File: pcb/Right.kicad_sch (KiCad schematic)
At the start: 51 parts

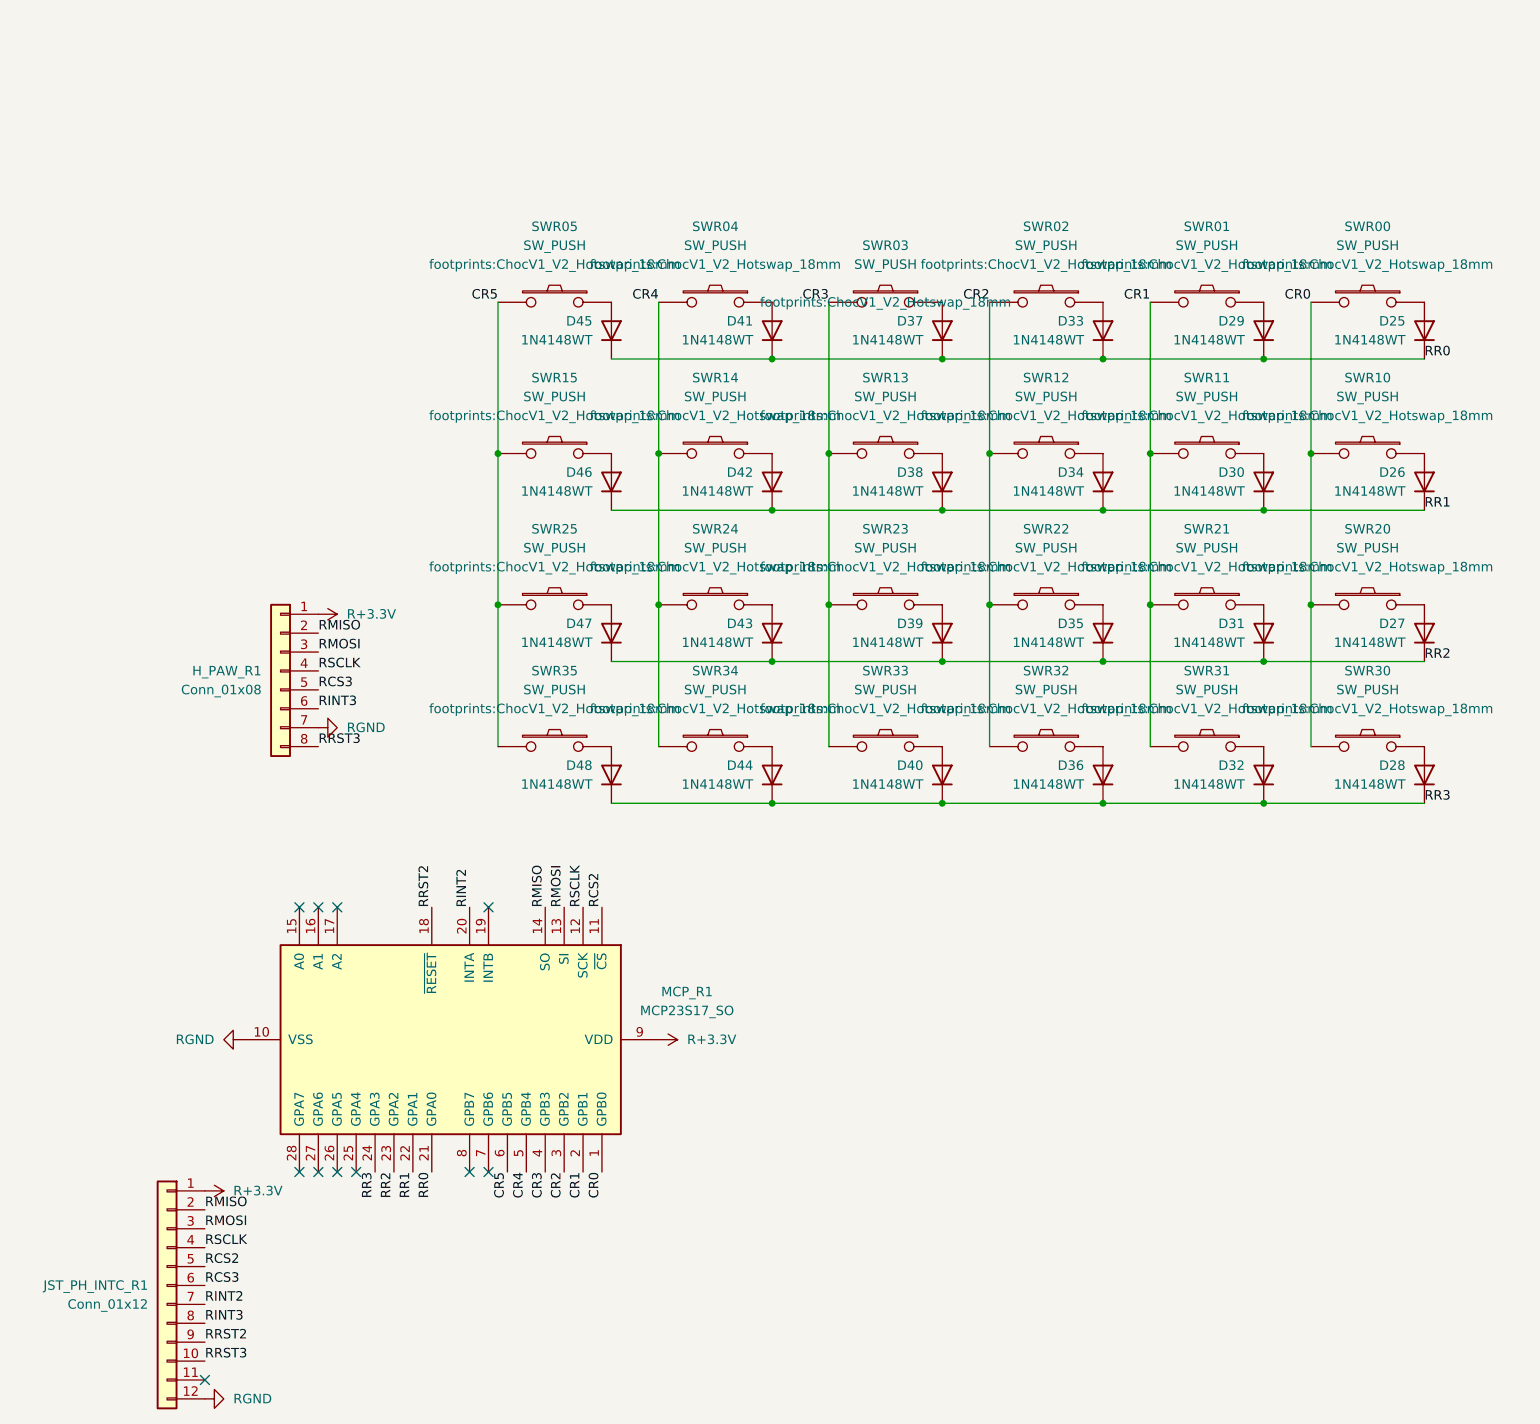
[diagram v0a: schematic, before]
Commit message: Clean up folder structure.
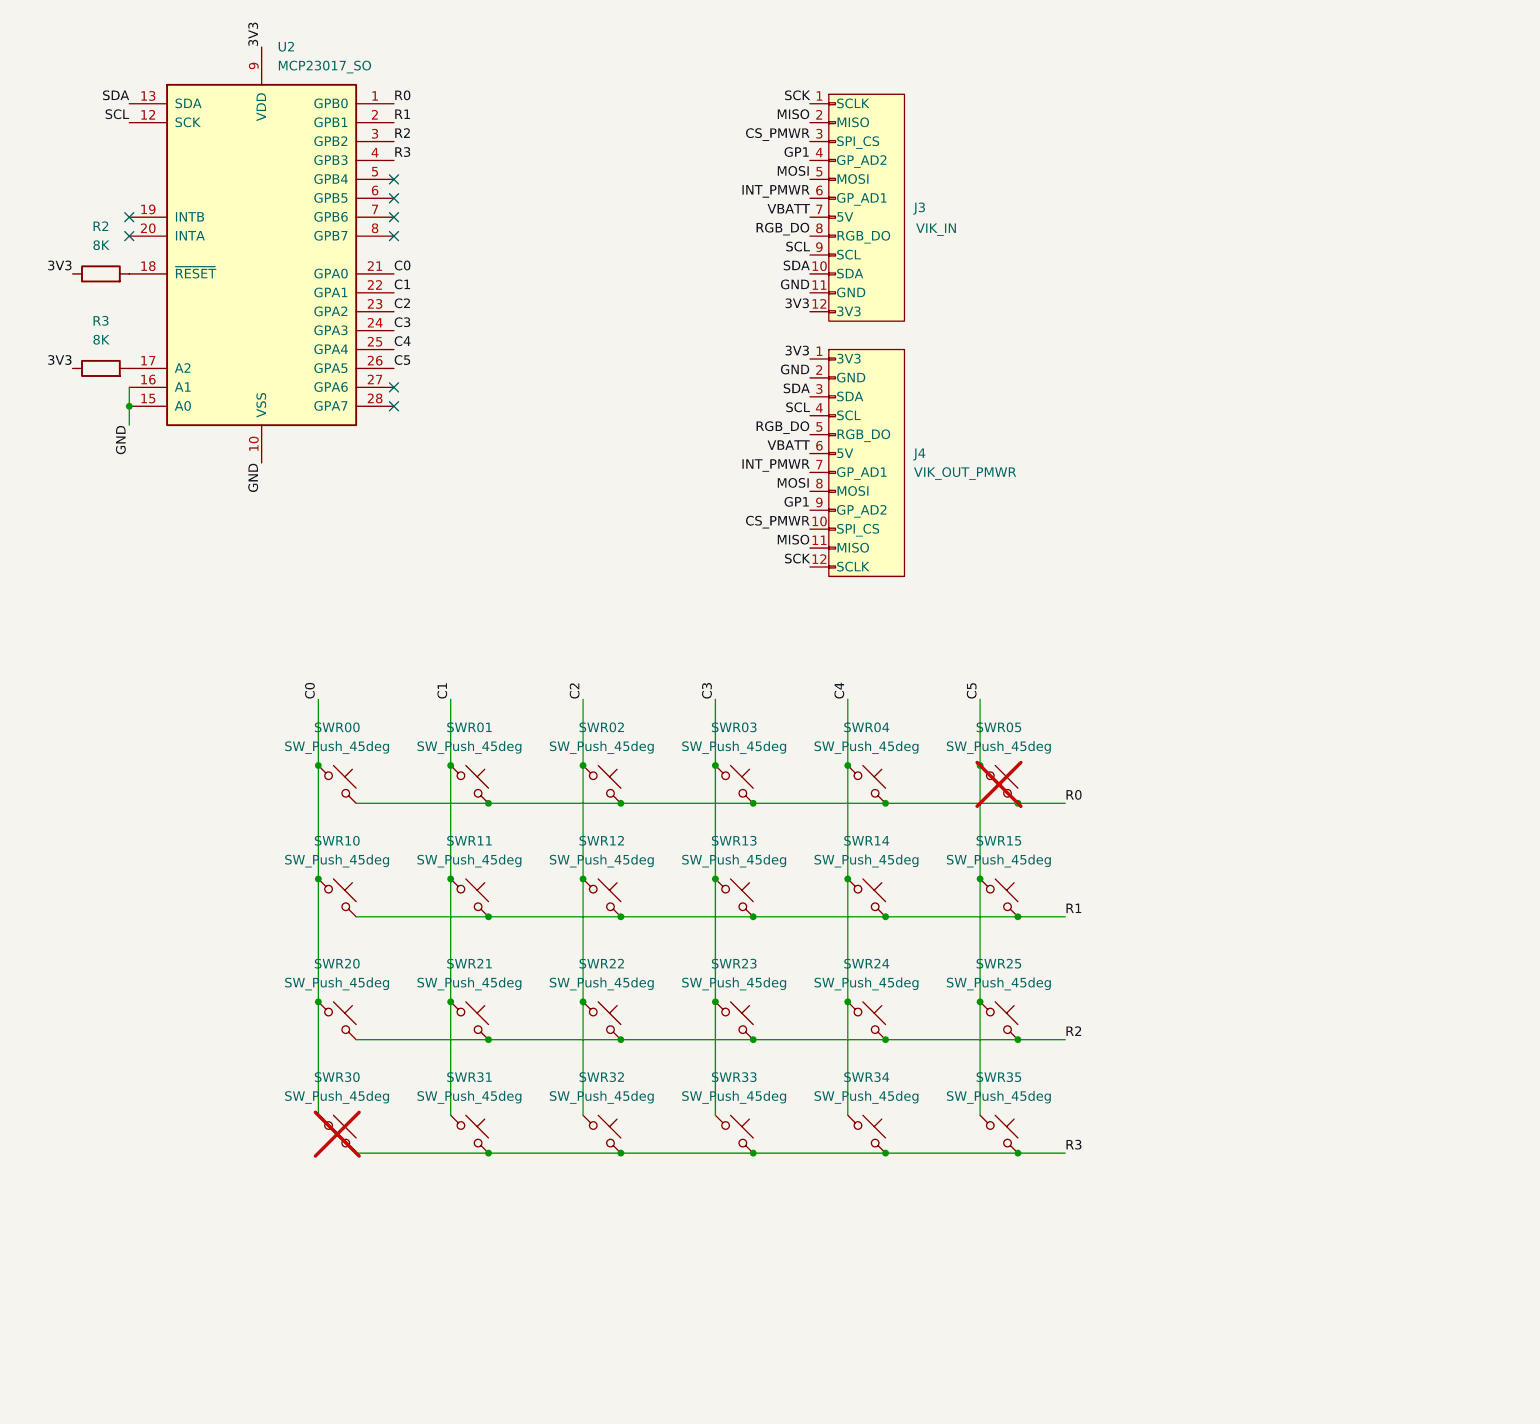
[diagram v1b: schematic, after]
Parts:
- removed D25, D26, D27, D28, D29, D30, D31, D32, D33, D34, D35, D36, D37, D38, D39, D40, D41, D42, D43, D44, D45, D46, D47, D48: 1N4148WT, Diode_SMD:D_SOD-523, symbol Diode:1N4148WT
- removed H_PAW_R1: Conn_01x08, Connector_PinHeader_2.54mm:PinHeader_1x08_P2.54mm_Horizontal, symbol Connector_Generic:Conn_01x08
- removed JST_PH_INTC_R1: Conn_01x12, Connector_JST:JST_PH_S12B-PH-K_1x12_P2.00mm_Horizontal, symbol Connector_Generic:Conn_01x12
- removed MCP_R1: MCP23S17_SO, Package_SO:SOIC-28W_7.5x17.9mm_P1.27mm, symbol Interface_Expansion:MCP23S17_SO
- removed SWR00, SWR01, SWR02, SWR03, SWR04, SWR05, SWR10, SWR11, SWR12, SWR13, SWR14, SWR15, SWR20, SWR21, SWR22, SWR23, SWR24, SWR25, SWR30, SWR31, SWR32, SWR33, SWR34, SWR35: SW_PUSH, footprints:ChocV1_V2_Hotswap_18mm, symbol kbd:SW_PUSH
- added J3: VIK_IN, Connector_JST:JST_PH_S12B-PH-K_1x12_P2.00mm_Horizontal, symbol vik:vik-module-connector
- added J4: VIK_OUT_PMWR, vik:vik-keyboard-connector-horizontal, symbol vik:vik-keyboard-connector
- added R2, R3: 8K, Resistor_SMD:R_0805_2012Metric_Pad1.20x1.40mm_HandSolder, symbol Device:R
- added SWR00, SWR01, SWR02, SWR03, SWR04, SWR10, SWR11, SWR12, SWR13, SWR14, SWR15, SWR20, SWR21, SWR22, SWR23, SWR24, SWR25, SWR31, SWR32, SWR33, SWR34, SWR35: SW_Push_45deg, footprints:ChocV1_V2_Hotswap, symbol Switch:SW_Push_45deg
- added SWR05, SWR30: SW_Push_45deg, symbol Switch:SW_Push_45deg
- added U2: MCP23017_SO, Package_SO:SOIC-28W_7.5x17.9mm_P1.27mm, symbol Interface_Expansion:MCP23017_SO
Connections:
- new net: R2.2, U2.18 (~{RESET})
- new net: R3.2, U2.17 (A2)
- new net 3V3: J3.12 (3V3), J4.1 (3V3), R2.1, R3.1, U2.9 (VDD)
- new net C0: SWR00.1, SWR10.1, SWR20.1, SWR30.1, U2.21 (GPA0)
- new net C1: SWR01.1, SWR11.1, SWR21.1, SWR31.1, U2.22 (GPA1)
- new net C2: SWR02.1, SWR12.1, SWR22.1, SWR32.1, U2.23 (GPA2)
- new net C3: SWR03.1, SWR13.1, SWR23.1, SWR33.1, U2.24 (GPA3)
- new net C4: SWR04.1, SWR14.1, SWR24.1, SWR34.1, U2.25 (GPA4)
- new net C5: SWR05.1, SWR15.1, SWR25.1, SWR35.1, U2.26 (GPA5)
- new net CS_PMWR: J3.3 (SPI_CS), J4.10 (SPI_CS)
- new net GND: J3.11 (GND), J4.2 (GND), U2.10 (VSS), U2.15 (A0), U2.16 (A1)
- new net GP1: J3.4 (GP_AD2), J4.9 (GP_AD2)
- new net INT_PMWR: J3.6 (GP_AD1), J4.7 (GP_AD1)
- new net MISO: J3.2 (MISO), J4.11 (MISO)
- new net MOSI: J3.5 (MOSI), J4.8 (MOSI)
- new net R0: SWR00.2, SWR01.2, SWR02.2, SWR03.2, SWR04.2, SWR05.2, U2.1 (GPB0)
- new net R1: SWR10.2, SWR11.2, SWR12.2, SWR13.2, SWR14.2, SWR15.2, U2.2 (GPB1)
- new net R2: SWR20.2, SWR21.2, SWR22.2, SWR23.2, SWR24.2, SWR25.2, U2.3 (GPB2)
- new net R3: SWR30.2, SWR31.2, SWR32.2, SWR33.2, SWR34.2, SWR35.2, U2.4 (GPB3)
- new net RGB_DO: J3.8 (RGB_DO), J4.5 (RGB_DO)
- new net SCK: J3.1 (SCLK), J4.12 (SCLK)
- new net SCL: J3.9 (SCL), J4.4 (SCL), U2.12 (SCK)
- new net SDA: J3.10 (SDA), J4.3 (SDA), U2.13 (SDA)
- new net VBATT: J3.7 (5V), J4.6 (5V)
- no-connect marks 11 -> 8
